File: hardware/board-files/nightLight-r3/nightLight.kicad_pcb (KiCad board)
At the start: 2 copper layers, 85 x 85 mm, 46 parts, among them IC1 PAM2401SCADJ, IC2 MCP73123T-22SI_MF, J1 USB_C_Receptacle_PowerOnly_6P, J2 Conn_01x05_Pin, J3 Conn_01x03, J4 Conn_01x03, J5 Conn_01x03, J6 Conn_01x03, Q1 AO3400A, Q2 AO3401A, SW1 TILT, U8 ATtiny1614-SS

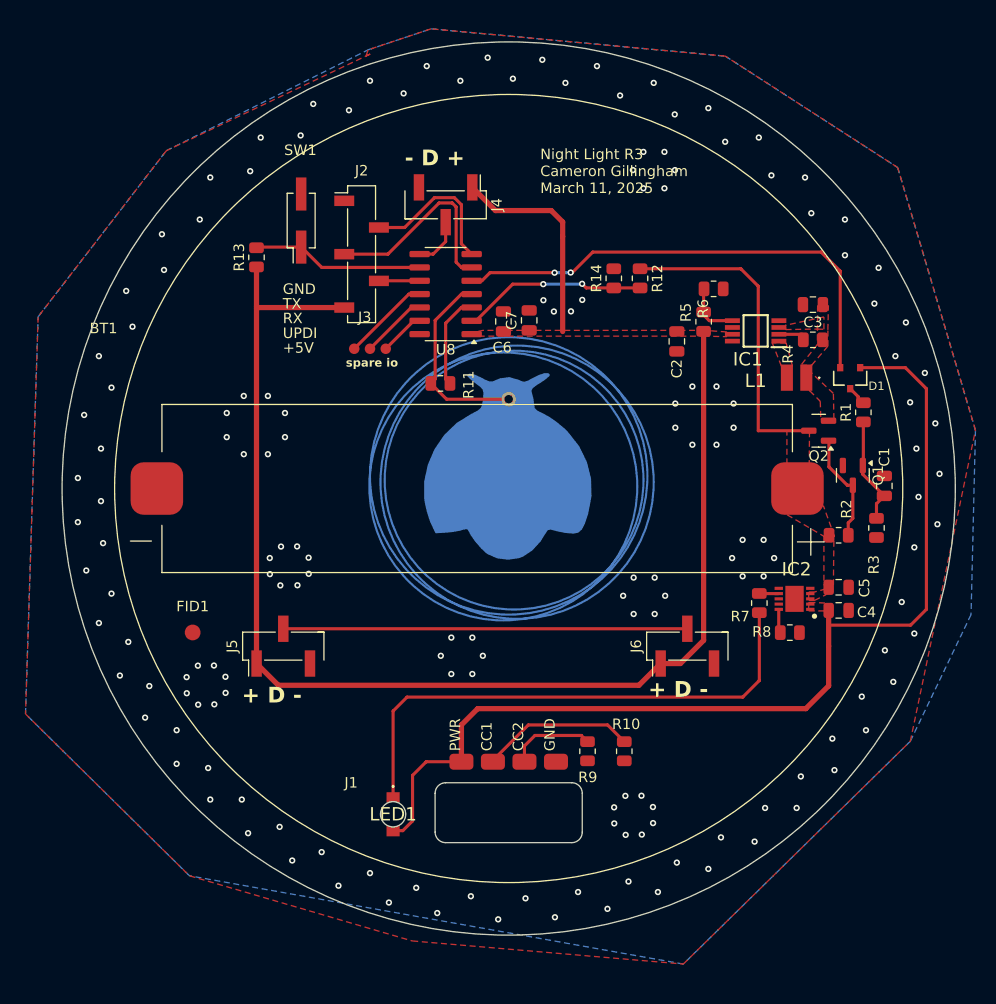
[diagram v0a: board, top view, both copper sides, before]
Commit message: rev3 done, errors eliminated
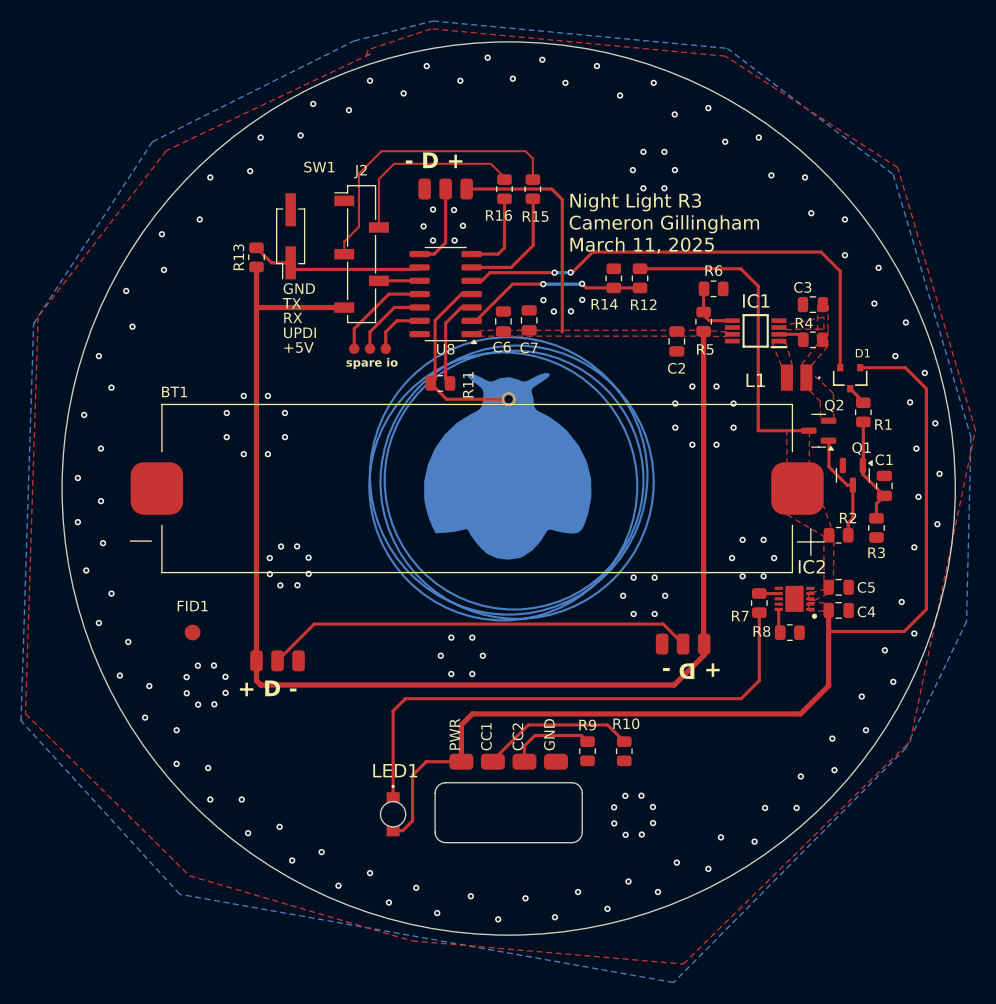
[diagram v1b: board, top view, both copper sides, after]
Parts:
- added R15: 0, Resistor_SMD:R_0805_2012Metric, F.Cu at (152.3, 71.5)
- added R16: 0, Resistor_SMD:R_0805_2012Metric, F.Cu at (149.6, 71.5)
- J4, J5, J6: footprint Connector_PinHeader_2.54mm:PinHeader_1x03_P2.54mm_Vertical_SMD_Pin1Left -> myFootprintDesigns:fairy_conn
- moved SW1 1.80 mm to (129.2, 76.0)
- moved J5 1.50 mm to (128.0, 116.4), turned to 0 degrees
- moved J4 1.50 mm to (144.0, 71.5), turned to 180 degrees
- moved J6 0.45 mm to (166.6, 114.8), turned to 180 degrees
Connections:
- J2 pad 2: /MCU/TX -> Net-(J2-Pin_2)
- J2 pad 3: /MCU/RX -> Net-(J2-Pin_3)
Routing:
- net Net-(J2-Pin_3): track 0.00 -> 27.9 mm
- net Net-(J2-Pin_2): track 0.00 -> 17.7 mm
- net /MCU/RX: track 19.8 -> 11.3 mm
- net /MCU/TX: track 14.4 -> 8.26 mm
- net /MCU/LED_DATA: track 4.81 -> 8.99 mm
- net +5V: track 141.1 -> 144.5 mm
- net Net-(J5-Pin_2): track 38.4 -> 40.8 mm
- net /MCU/PA_1: track 8.38 -> 9.49 mm
- net /MCU/PA_3: track 4.33 -> 5.26 mm
- net /MCU/PA_2: track 6.35 -> 7.29 mm
- net GND: vias 163 -> 169
